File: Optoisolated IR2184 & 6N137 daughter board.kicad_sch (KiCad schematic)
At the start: 16 parts, among them J1 Screw_Terminal_01x08, U1 6N137, U2 IR2184, U3 ADP7118ACPZN

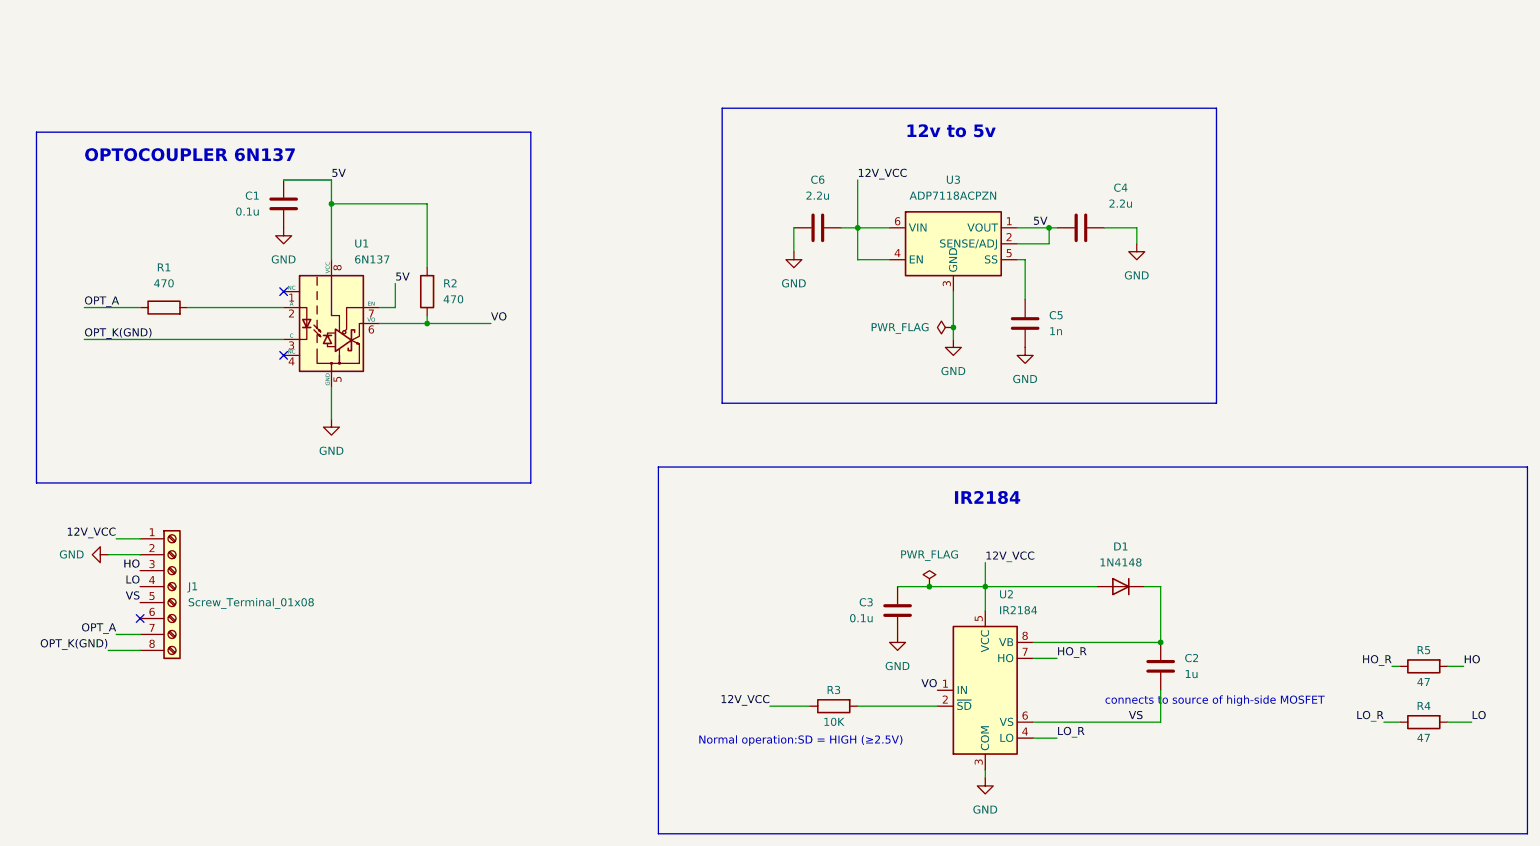
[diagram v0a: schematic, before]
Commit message: PCB LAYOUT
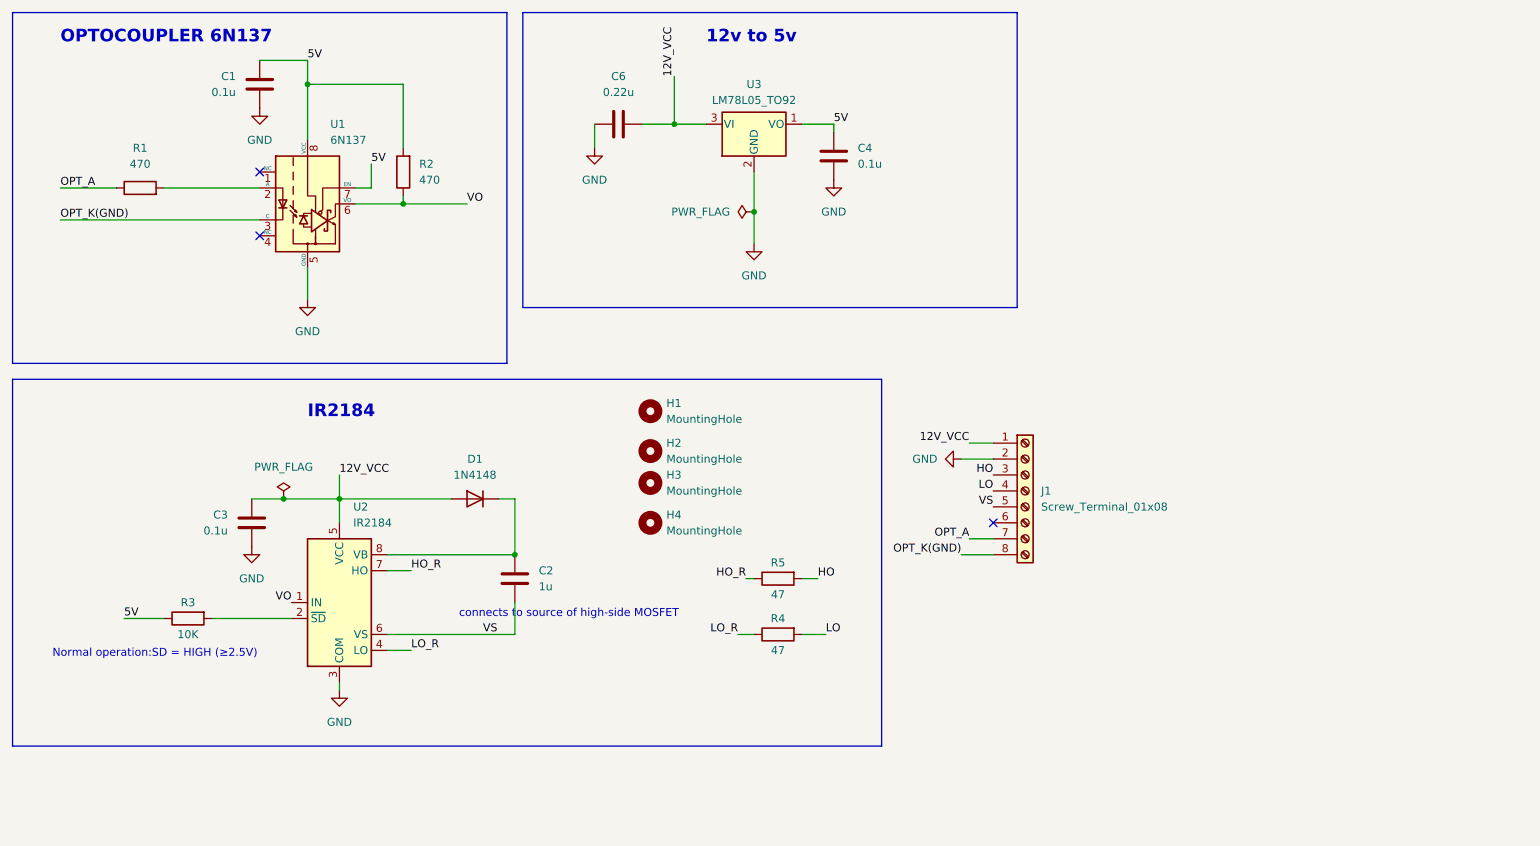
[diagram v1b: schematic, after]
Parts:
- removed C5: 1n, Capacitor_SMD:C_0805_2012Metric_Pad1.18x1.45mm_HandSolder, symbol Device:C
- removed U3: ADP7118ACPZN, Package_CSP:LFCSP-6-1EP_2x2mm_P0.65mm_EP1x1.6mm, symbol Regulator_Linear:ADP7118ACPZN
- added H1, H2, H3, H4: MountingHole, MountingHole:MountingHole_3.2mm_M3, symbol Mechanical:MountingHole
- added U3: LM78L05_TO92, Package_TO_SOT_THT:TO-220F-3_Vertical, symbol Regulator_Linear:LM78L05_TO92
- C1, C3: footprint Capacitor_SMD:C_0805_2012Metric_Pad1.18x1.45mm_HandSolder -> Capacitor_THT:C_Disc_D5.0mm_W2.5mm_P2.50mm; Manufacturer Vishay -> kemet; Manufacturer Part Number VJ0805Y104JXAAT -> C326C104K5R5TA; Package 0805 -> Radial; Supplier Part Number 720-2029-1-ND -> 399-9824-ND
- C2: footprint Capacitor_SMD:C_1206_3216Metric_Pad1.33x1.80mm_HandSolder -> Capacitor_THT:C_Disc_D5.0mm_W2.5mm_P2.50mm; Manufacturer KYOCERA AVX -> Murata Electronics; Manufacturer Part Number 12065C105JAT2A -> RDEC71E105K0P1H03B; Package 1206 -> Radial; Supplier Part Number 478-KGM31HR71H105JUCT-ND -> RDEC71E105K0P1H03B-ND; Voltage 50v -> 25v
- C4: value 2.2u -> 0.1u; footprint Capacitor_SMD:C_0805_2012Metric_Pad1.18x1.45mm_HandSolder -> Capacitor_THT:C_Disc_D5.0mm_W2.5mm_P2.50mm; Manufacturer Murata Electronics -> kemet; Manufacturer Part Number GRM21BR71C225KA12L -> C326C104K5R5TA; Package 0805 -> Radial; Supplier Part Number 490-3906-6-ND -> 399-9824-ND; Voltage 16v -> 50v
- C6: value 2.2u -> 0.22u; footprint Capacitor_SMD:C_0805_2012Metric_Pad1.18x1.45mm_HandSolder -> Capacitor_THT:C_Disc_D5.0mm_W2.5mm_P2.50mm; Manufacturer Murata Electronics -> Vishay; Manufacturer Part Number GRM21BR71C225KA12L -> K224Z15Y5VF5TL2; Package 0805 -> Radial; Supplier Part Number 490-3906-6-ND -> BC1161TR-ND; Voltage 16v -> 50v
- D1: footprint Diode_SMD:D_SOD-123 -> Diode_THT:D_DO-35_SOD27_P7.62mm_Horizontal; Manufacturer Part Number 1N4148W-E3-08 -> 1N4148-TAP; Package SOD-123 -> DO-35 Axial; Supplier Part Number 1N4148W-E3-08CT-ND -> 1N4148-TAPCT-ND
- R1, R2: footprint Resistor_SMD:R_0805_2012Metric_Pad1.20x1.40mm_HandSolder -> Resistor_THT:R_Axial_DIN0207_L6.3mm_D2.5mm_P7.62mm_Horizontal; Manufacturer Part Number CRG0805F470R -> CFR16J470R; Package 0805 -> Radial; Supplier Part Number A106063CT-ND -> A105933CT-ND
- R3: footprint Resistor_SMD:R_0805_2012Metric_Pad1.20x1.40mm_HandSolder -> Resistor_THT:R_Axial_DIN0207_L6.3mm_D2.5mm_P7.62mm_Horizontal; Manufacturer Part Number CRG0805F10K/10 -> CFR16J10K; Package 0805 -> Radial; Supplier Part Number A126332CT-ND -> A104668CT-ND
- R4, R5: footprint Resistor_SMD:R_1206_3216Metric_Pad1.30x1.75mm_HandSolder -> Resistor_THT:R_Axial_DIN0207_L6.3mm_D2.5mm_P7.62mm_Horizontal; Manufacturer Part Number CRGP1206F47R -> LR0204F47R; Package 1206 -> Radial; Supplier Part Number A130522CT-ND -> LR0204F47R-ND
- U2: footprint Package_DIP:DIP-8_W8.89mm_SMDSocket_LongPads -> Package_DIP:DIP-8_W7.62mm; Supplier Part Number IR2184SPBF-ND -> IR2184PBF-ND
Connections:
- net 12V_VCC: now also U3.3 (VI); no longer R3.1
- net 5V: now also R3.1, U3.1 (VO)
- net GND: now also U3.2 (GND)
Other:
- moved on the sheet: C1, C2, C3, C6, D1, J1, R1, R2, R3, R4, R5, U1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
